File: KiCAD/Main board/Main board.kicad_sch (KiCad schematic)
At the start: 5 parts, among them J1 Conn_01x03, J2 Conn_01x03, J3 Conn_01x02, J4 Conn_01x03, J5 Conn_01x02

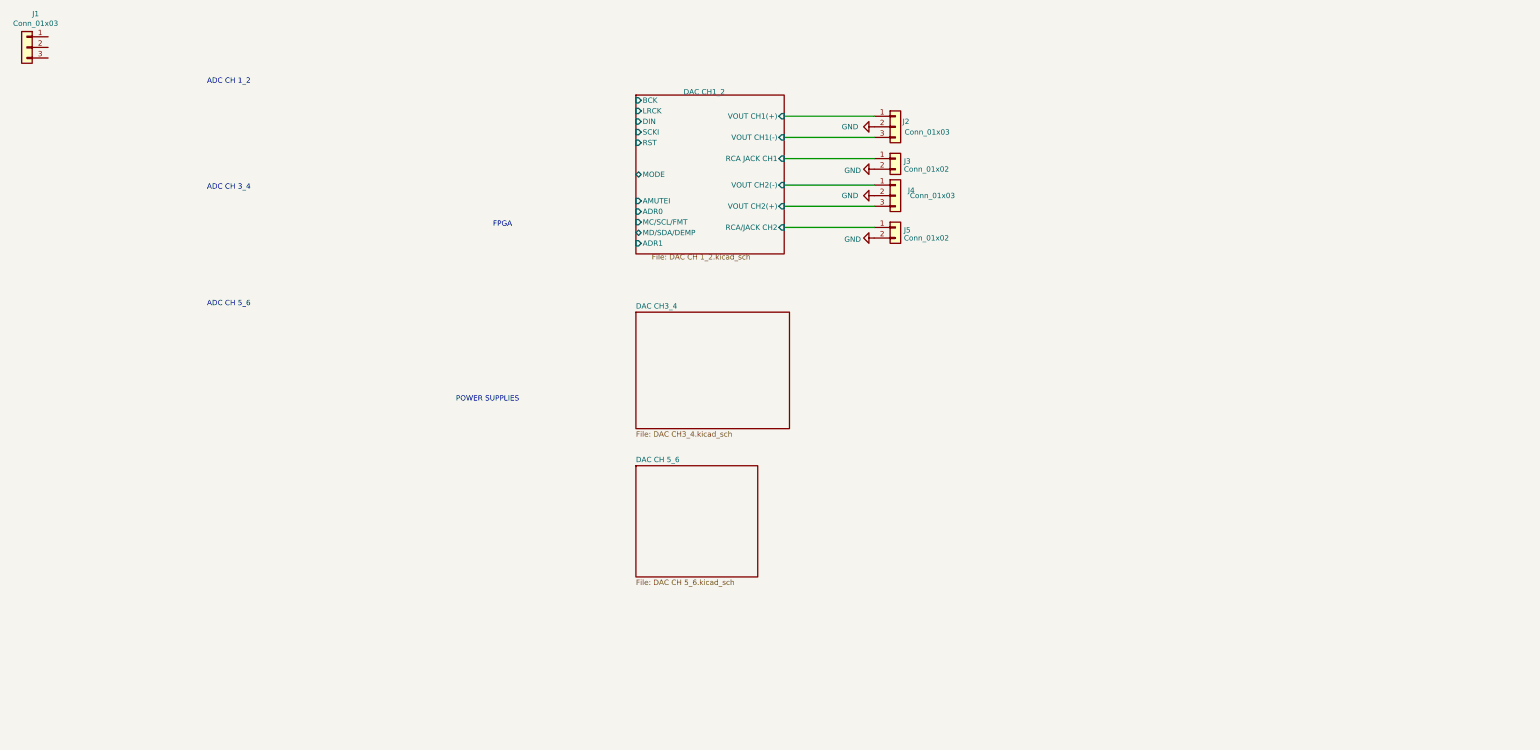
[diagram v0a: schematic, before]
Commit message: Updated BACK-END
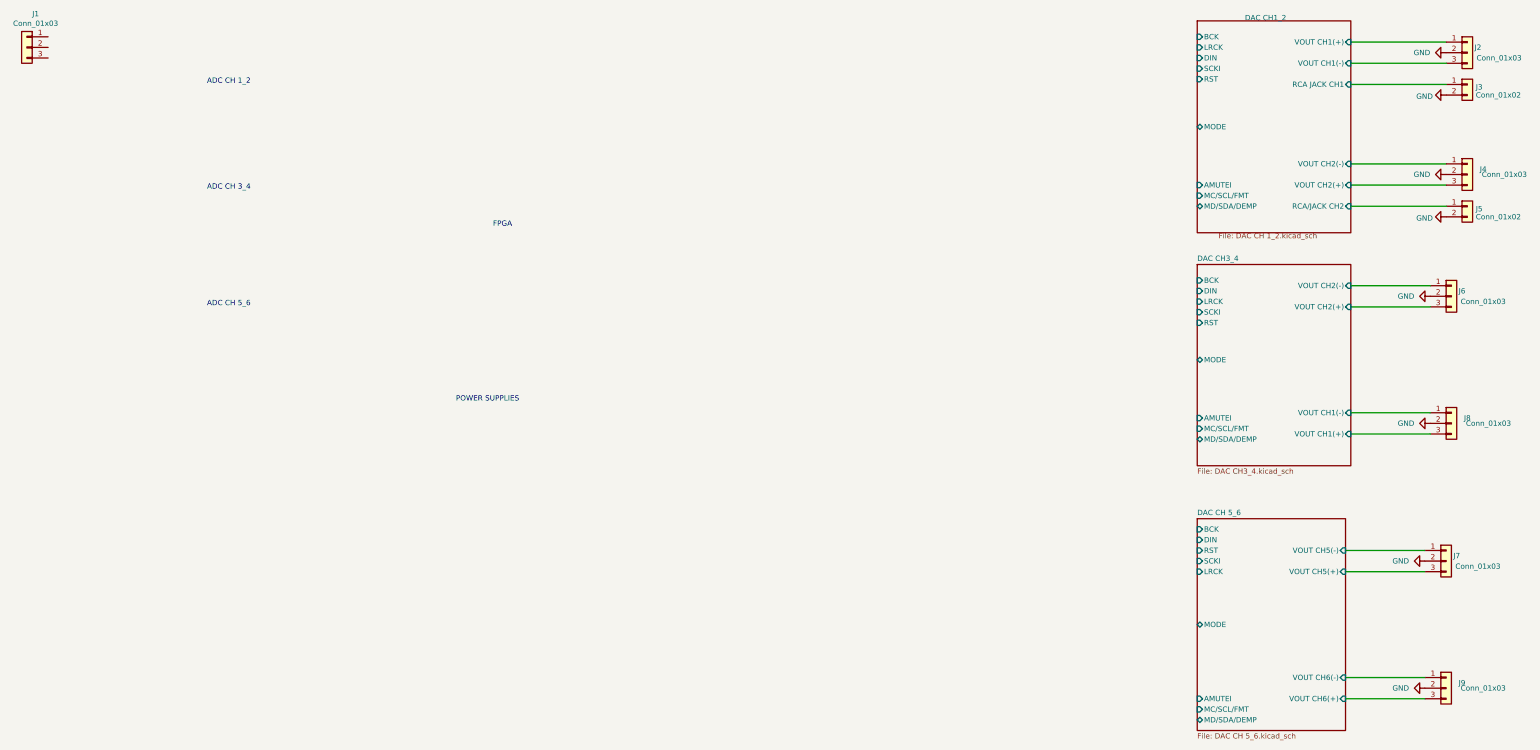
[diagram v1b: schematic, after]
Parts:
- added J6, J7, J8, J9: Conn_01x03, Connector_JST:JST_PH_B3B-PH-K_1x03_P2.00mm_Vertical, symbol Connector_Generic:Conn_01x03
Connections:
- net GND: now also J6.2 (Pin_2), J7.2 (Pin_2), J8.2 (Pin_2), J9.2 (Pin_2)
- new net DAC CH 5_6/VOUT CH5(+): J7.3 (Pin_3)
- new net DAC CH 5_6/VOUT CH5(-): J7.1 (Pin_1)
- new net DAC CH 5_6/VOUT CH6(+): J9.3 (Pin_3)
- new net DAC CH 5_6/VOUT CH6(-): J9.1 (Pin_1)
- new net DAC CH3_4/VOUT CH1(+): J8.3 (Pin_3)
- new net DAC CH3_4/VOUT CH1(-): J8.1 (Pin_1)
- new net DAC CH3_4/VOUT CH2(+): J6.3 (Pin_3)
- new net DAC CH3_4/VOUT CH2(-): J6.1 (Pin_1)
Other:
- sheet DAC CH 5_6 ports: added AMUTEI, BCK, DIN, LRCK, MC/SCL/FMT, MD/SDA/DEMP, MODE, RST, SCKI, VOUT CH5(+), VOUT CH5(-), VOUT CH6(+), VOUT CH6(-); removed none
- sheet DAC CH1_2 ports: added none; removed ADR0, ADR1
- sheet DAC CH3_4 ports: added AMUTEI, BCK, DIN, LRCK, MC/SCL/FMT, MD/SDA/DEMP, MODE, RST, SCKI, VOUT CH1(+), VOUT CH1(-), VOUT CH2(+), VOUT CH2(-); removed none
- moved on the sheet: J2, J3, J4, J5
